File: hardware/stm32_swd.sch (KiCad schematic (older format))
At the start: 2 parts

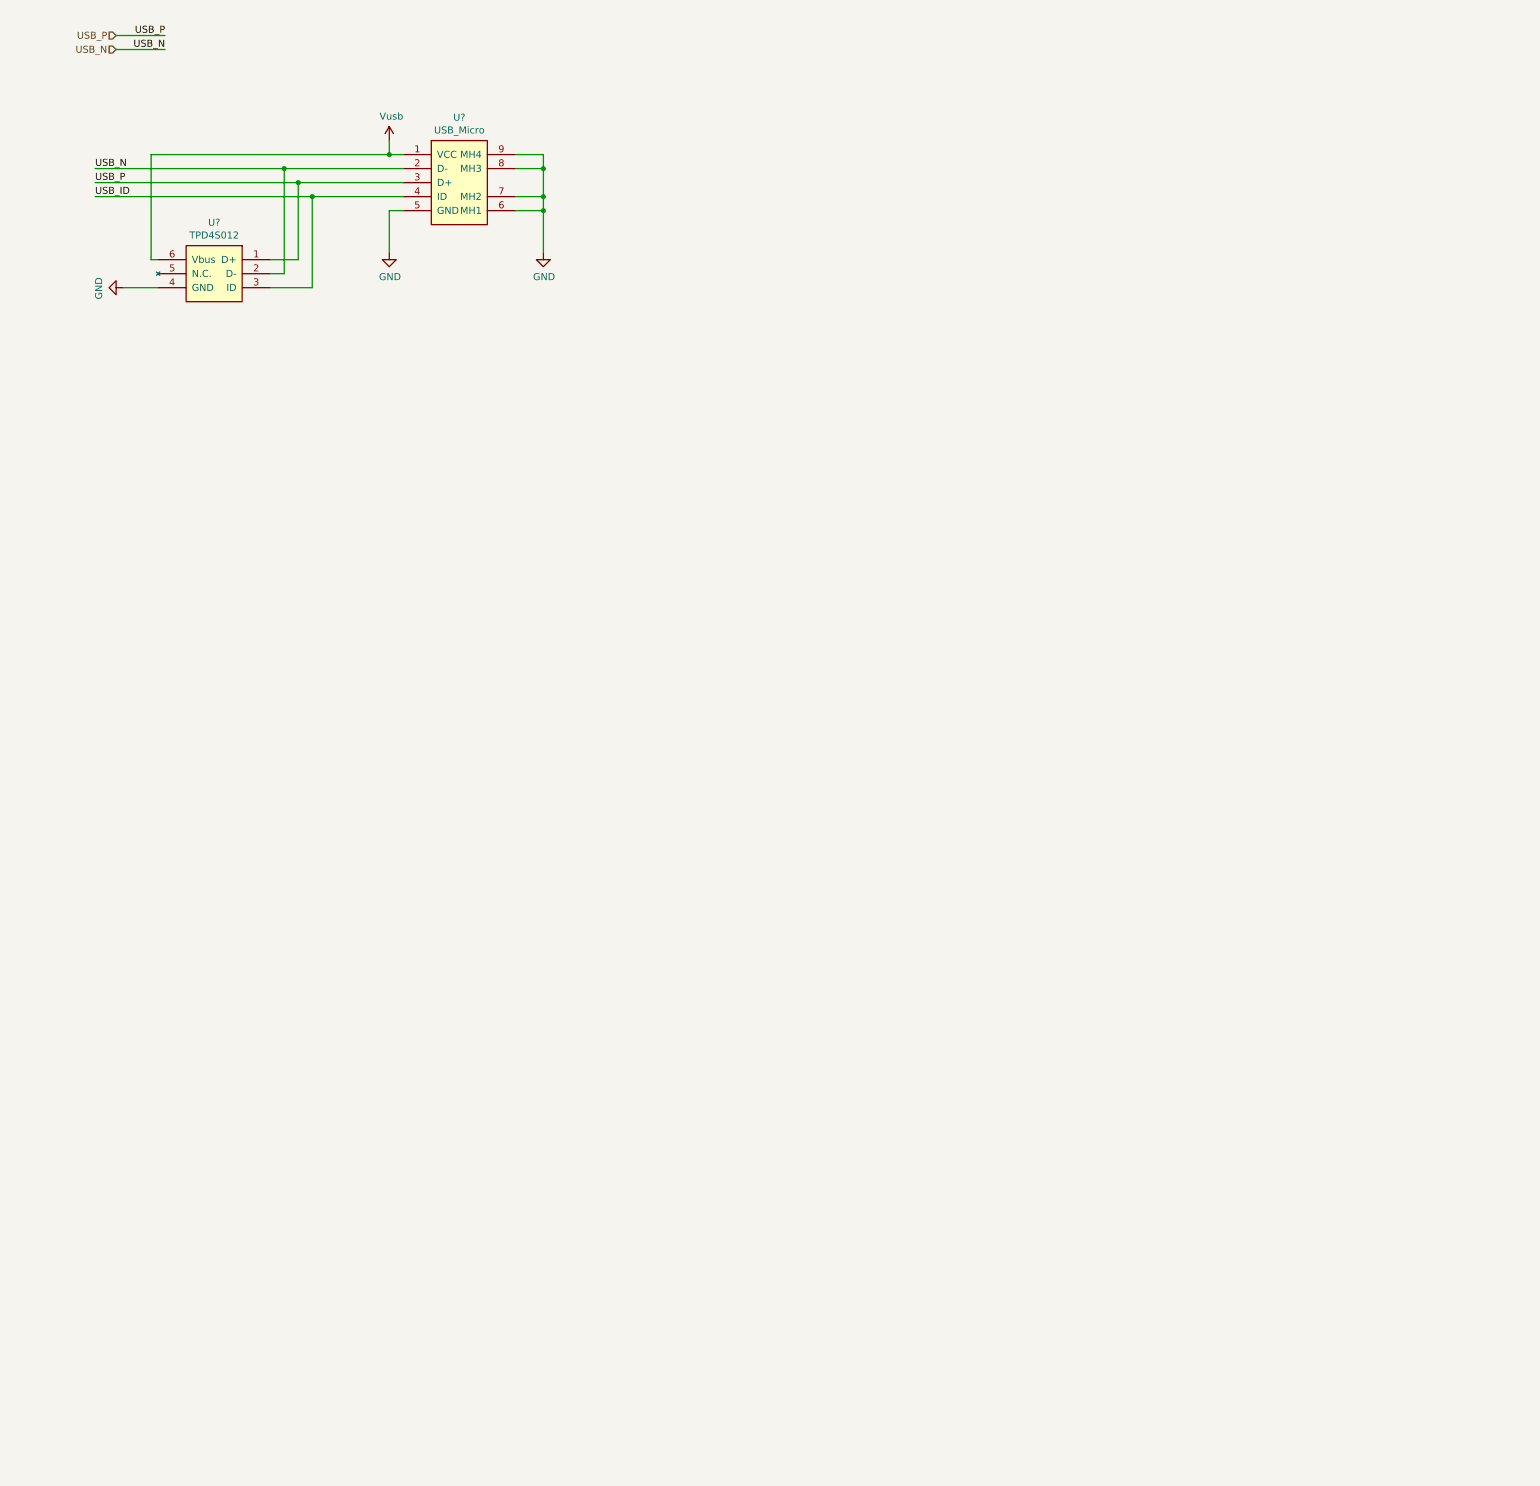
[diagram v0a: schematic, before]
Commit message: update,
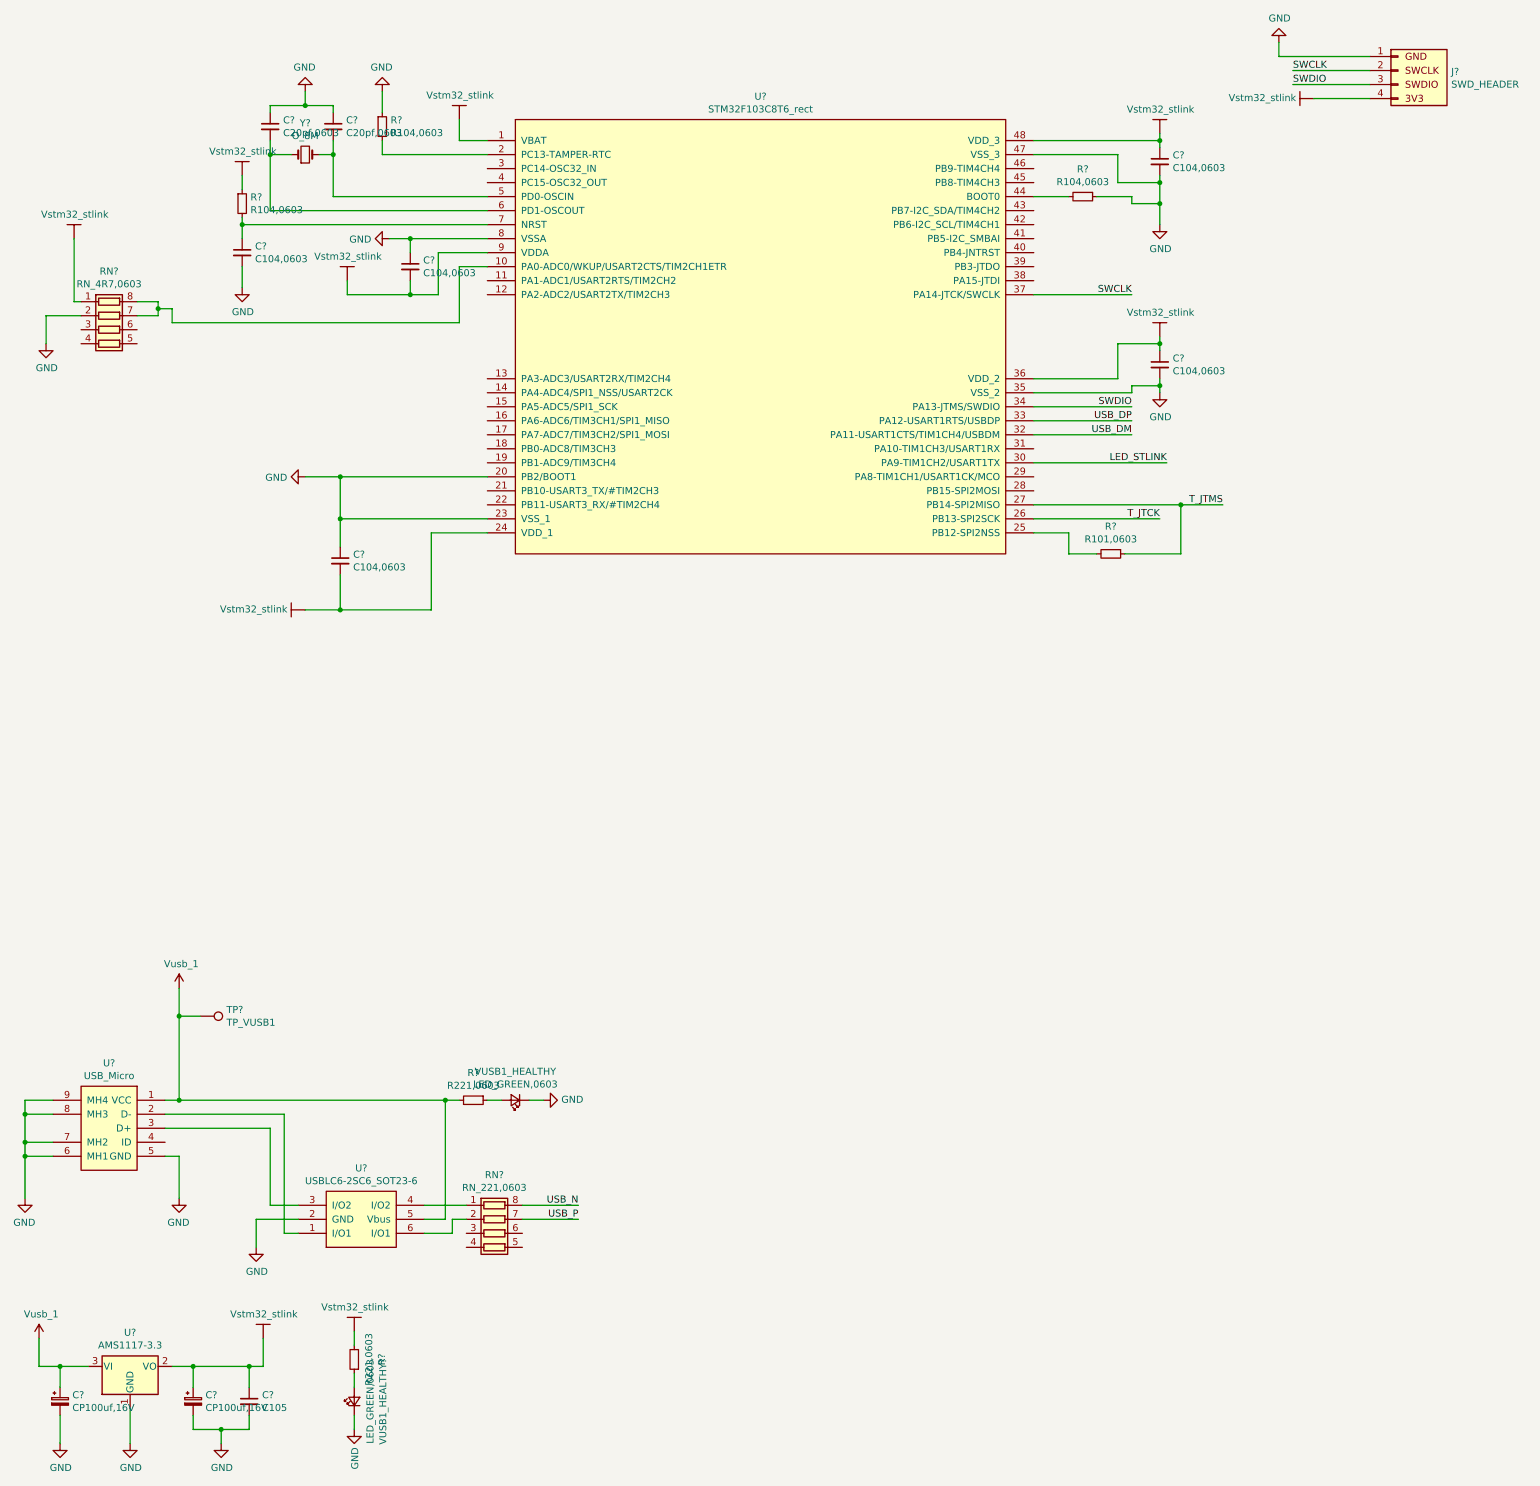
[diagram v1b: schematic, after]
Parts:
- removed U?: USB_Micro, footprint-lib:USB_Micro-B_Molex-105017-0001, symbol taobao-components:USB_Micro
- removed U?: TPD4S012, footprints-lib:TPD4S012, symbol taobao-components:TPD4S012
- added C?: C105, Capacitor_SMD:C_0603_1608Metric_Pad1.05x0.95mm_HandSolder, symbol taobao-c:C105
- added C? (x2): CP100uf,16V, Capacitor_SMD:CP_Elec_6.3x5.3, symbol taobao-cp:CP100uf,16V
- added C? (x2): C20pf,0603, Capacitor_SMD:C_0603_1608Metric_Pad1.05x0.95mm_HandSolder, symbol taobao-c:C20pf,0603
- added C? (x5): C104,0603, Capacitor_SMD:C_0603_1608Metric_Pad1.05x0.95mm_HandSolder, symbol taobao-c:C104,0603
- added J?: SWD_HEADER, footprint-lib:BLUEPILL_SWD, symbol taobao-components:BLUEPILL_SWD
- added R? (x2): R221,0603, Resistor_SMD:R_0603_1608Metric_Pad1.05x0.95mm_HandSolder, symbol taobao-r:R221,0603
- added R? (x3): R104,0603, Resistor_SMD:R_0603_1608Metric_Pad1.05x0.95mm_HandSolder, symbol taobao-r:R104,0603
- added R?: R101,0603, Resistor_SMD:R_0603_1608Metric_Pad1.05x0.95mm_HandSolder, symbol taobao-r:R101,0603
- added RN?: RN_221,0603, Resistor_SMD:R_Array_Concave_4x0603, symbol taobao-rpack:RN_221,0603
- added RN?: RN_4R7,0603, Resistor_SMD:R_Array_Concave_4x0603, symbol taobao-rpack:RN_4R7,0603
- added TP?: TP_VUSB1, TestPoint:TestPoint_THTPad_D2.0mm_Drill1.0mm, symbol my_testpoint:TestPoint_2mm
- added U?: AMS1117-3.3, Package_TO_SOT_SMD:SOT-223-3_TabPin2, symbol Regulator_Linear:AMS1117-3.3
- added U?: STM32F103C8T6_rect, footprint-lib:STM32F103C8T6, symbol taobao-components:STM32F103C8T6_rect
- added U?: USB_Micro, footprint-lib:USB_Micro-B_Molex-105017-0001, symbol taobao-components:USB_Micro
- added U?: USBLC6-2SC6_SOT23-6, footprints-lib:USBLC6-2, symbol taobao-components:USBLC6-2SC6_SOT23-6
- added VUSB1_HEALTHY, VUSB1_HEALTHY?: LED_GREEN,0603, footprint-lib:LED_0603_1608Metric, symbol taobao-led:LED_GREEN,0603
- added Y?: O_8M, Crystal:Crystal_HC49-4H_Vertical, symbol taobao-osc:O_8M
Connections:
- net GND: now also C?.1, C?.1, C?.1, C?.1, C?.2, C?.2, C?.2, C?.2, C?.2, C?.2, J?.1 (Pin_1), R?.1, R?.1, RN?.2 (R2.1), U?.1 (GND), U?.2 (GND), U?.20 (PB2/BOOT1), U?.23 (VSS_1), U?.35 (VSS_2), U?.47 (VSS_3), U?.5 (GND), U?.6 (MH1), U?.7 (MH2), U?.8 (MH3), U?.8 (VSSA), U?.9 (MH4), VUSB1_HEALTHY.1 (K), VUSB1_HEALTHY?.1 (K)
- net USB_N: now also RN?.8 (R1.2)
- net USB_P: now also RN?.7 (R2.2)
- new net: RN?.7 (R2.2), RN?.8 (R1.2), U?.10 (PA0-ADC0/WKUP/USART2CTS/TIM2CH1ETR)
- new net: R?.2, U?.2 (PC13-TAMPER-RTC)
- new net: R?.2, U?.25 (PB12-SPI2NSS)
- new net: R?.2, U?.44 (BOOT0)
- new net: C?.2, U?.5 (PD0-OSCIN), Y?.2
- new net: C?.2, U?.6 (PD1-OSCOUT), Y?.1
- new net: C?.1, R?.2, U?.7 (NRST)
- new net: U?.1 (I/O1), U?.2 (D-)
- new net: U?.3 (D+), U?.3 (I/O2)
- new net: RN?.1 (R1.1), U?.4 (I/O2)
- new net: RN?.2 (R2.1), U?.6 (I/O1)
- new net: R?.1, VUSB1_HEALTHY.2 (A)
- new net: R?.1, VUSB1_HEALTHY?.2 (A)
- new net LED_STLINK: U?.30 (PA9-TIM1CH2/USART1TX)
- new net SWCLK: J?.2 (Pin_2), U?.37 (PA14-JTCK/SWCLK)
- new net SWDIO: J?.3 (Pin_3), U?.34 (PA13-JTMS/SWDIO)
- new net T_JTCK: U?.26 (PB13-SPI2SCK)
- new net T_JTMS: R?.1, U?.27 (PB14-SPI2MISO)
- new net USB_DM: U?.32 (PA11-USART1CTS/TIM1CH4/USBDM)
- new net USB_DP: U?.33 (PA12-USART1RTS/USBDP)
- new net Vstm32_stlink: C?.1, C?.1, C?.1, C?.1, C?.2, C?.2, J?.4 (Pin_4), R?.1, R?.2, RN?.1 (R1.1), U?.1 (VBAT), U?.2 (VO), U?.24 (VDD_1), U?.36 (VDD_2), U?.48 (VDD_3), U?.9 (VDDA)
- new net Vusb_1: C?.1, R?.2, TP?.1, U?.1 (VCC), U?.3 (VI), U?.5 (Vbus)
